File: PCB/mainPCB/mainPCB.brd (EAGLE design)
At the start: 187 x 85 mm, 129 parts, among them CN1 SDS-50J, CN2 SDS-50J, CN3 SDS-50J, CN4 SDS-50J, CN5 SDS-50J, CN6 SDS-50J, CN7 SDS-50J, CN8 SDS-50J, CON1 1776244-4, J2 RASPBERRYPI-40-PIN-GPIO, Q1 DMMT5401-7-F, T2 BC817, T3 BC817, T4 BC817, T5 BC817, T6 BC817, T7 BC817, T8 BC817, T9 BC817, U1 AT24C256C-SSHL-B, U11 SFH615A-07, U12 ALQ105, U13 SFH615A-07, U14 ALQ105, U15 SFH615A-07, U16 ALQ105, U17 SFH615A-07, U18 ALQ105, U19 SFH615A-07, U2 DMG2305UX-13SOT-23-M, U20 ALQ105, U3 SFH615A-07, U4 ALQ105, U5 SFH615A-07, U6 ALQ105, U7 SFH615A-07, U8 ALQ105

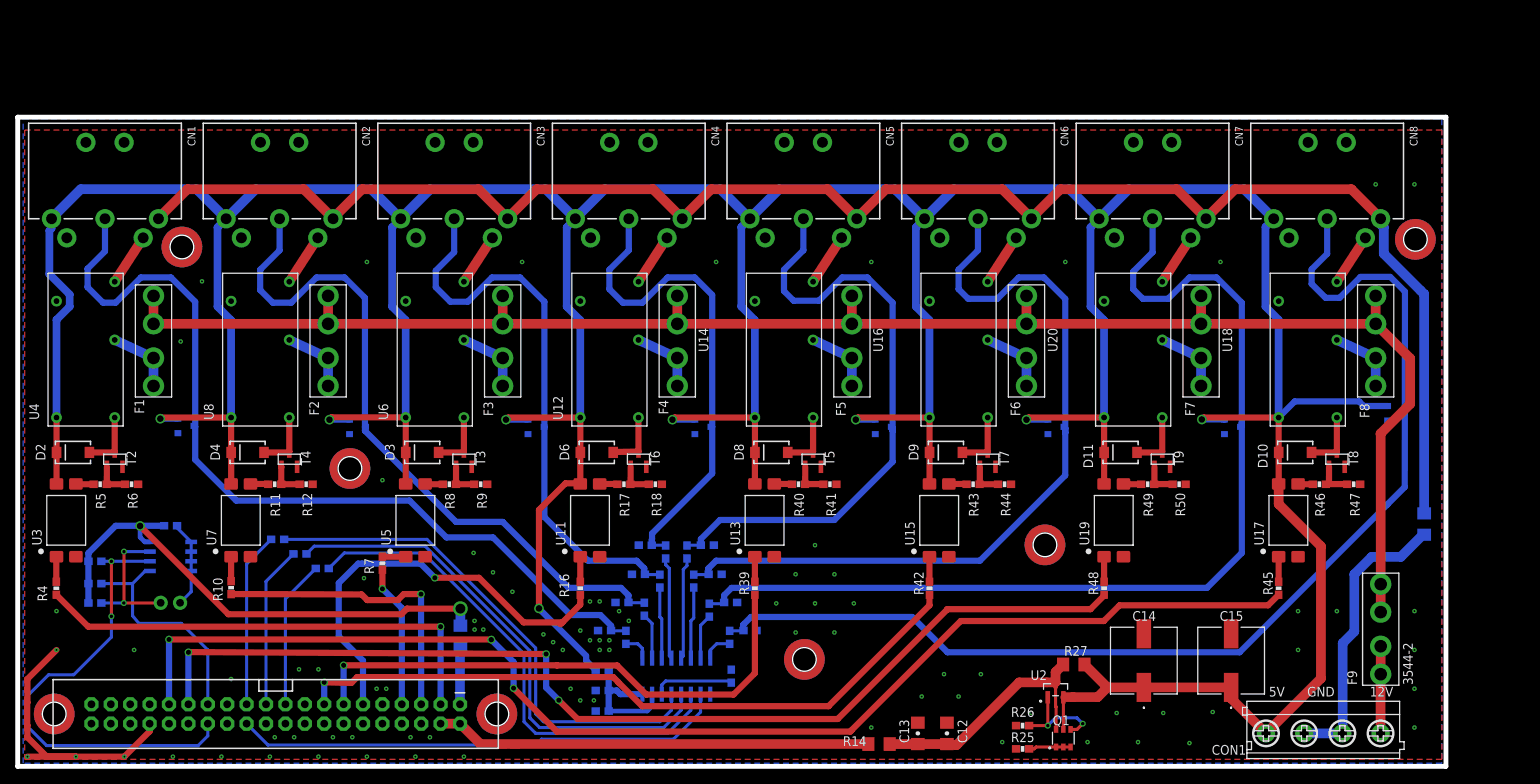
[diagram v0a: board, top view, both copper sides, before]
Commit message: Technically version 0.4. Sending it to JLCPCB for production.
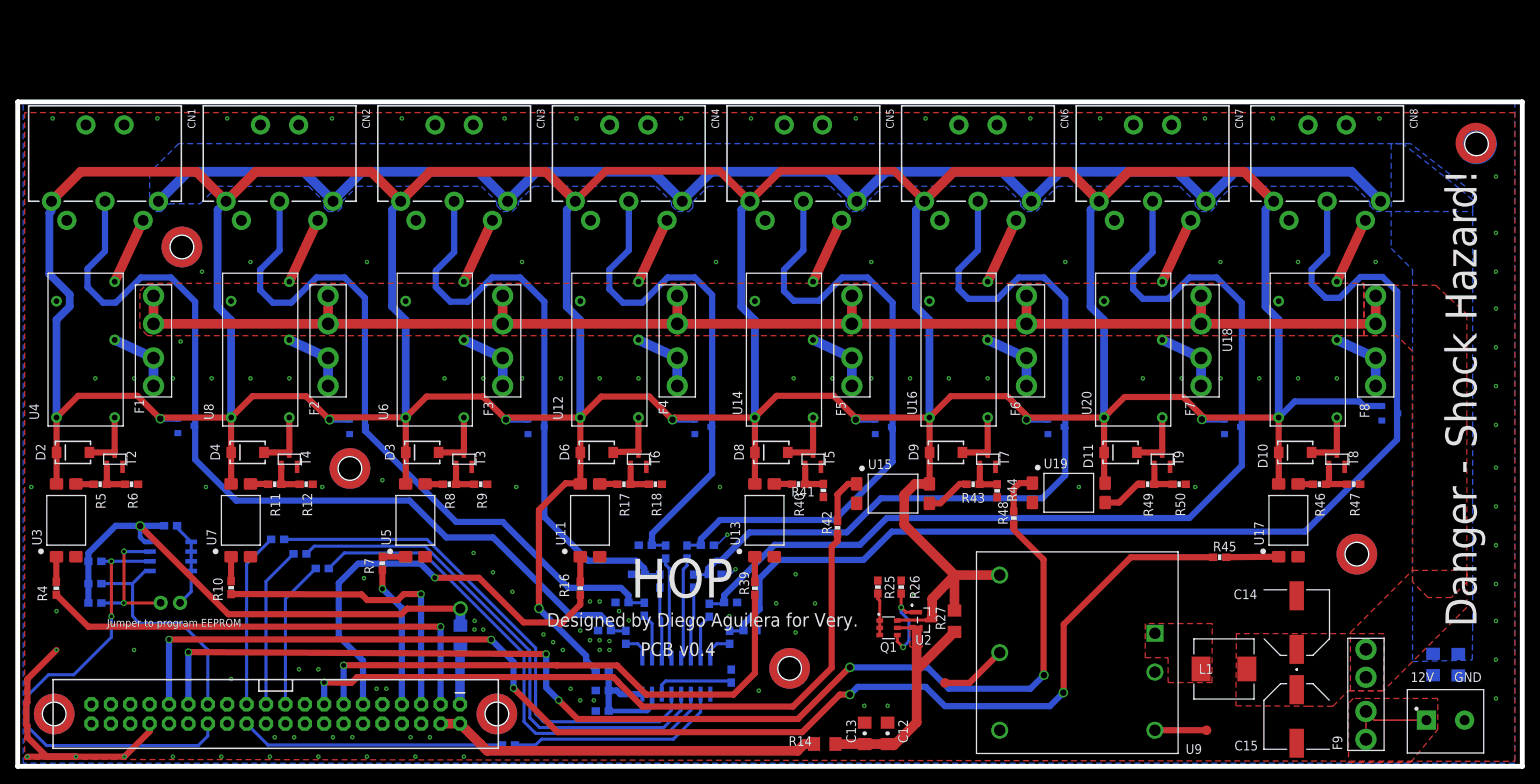
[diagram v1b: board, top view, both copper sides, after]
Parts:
- removed CON1: 1776244-4, lib:1776244-4
- added J1: 1935161, 1935161:PHOENIX_1935161
- added L1: DR73-1R0-R, DR73-1R0-R:DR73
- added R36: 0, SparkFun-Passives:1206
- added TP_ON/OFF, TP_TRIM: TEST-POINT3X5, SparkFun-Passives:PAD.03X.05
- added U9: S24SE05004PDFA, S24SE05004PDFA:CONV_S24SE05002PDFA
- C12, C13: value 10uF -> 1uF
- moved R25 28.4 mm to (112.6, 23.5), turned to 270 degrees
- moved Q1 27.1 mm to (114.0, 18.1), turned to 0 degrees
- moved R26 24.1 mm to (115.7, 23.5), turned to 270 degrees
- moved C14 20.6 mm to (167.5, 18.8)
- moved U2 19.6 mm to (118.6, 19.2), turned to 270 degrees
- moved R24 18.4 mm to (185.3, 13.3)
- moved R27 16.6 mm to (122.7, 19.0), turned to 270 degrees
- moved R48 15.0 mm to (130.4, 32.5)
- moved R42 14.4 mm to (107.3, 31.2)
- moved C15 11.3 mm to (167.5, 6.53), turned to 270 degrees
- moved F9 8.75 mm to (176.5, 9.42)
- moved R45 8.72 mm to (157.4, 27.4), turned to 0 degrees
- moved C12 7.77 mm to (113.9, 4.32)
- moved R14 7.11 mm to (105.7, 2.92)
- moved U15 6.98 mm to (114.6, 35.7), turned to 0 degrees
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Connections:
- removed net N$28: CON1.4, F9.P$1, F9.P$2
- new net N$30: TP_ON/OFF.P$1, U9.3
- new net N$52: L1.1, U9.1
- new net N$53: TP_TRIM.P$1, U9.5
- new net N$54: F9.P$1, F9.P$2, J1.1
- net 12V: now also C14.1, C15.1, L1.2
- net 5V: now also Q1.6, R27.1, U2.3, U9.6; no longer C14.1, C15.1, CON1.1, Q1.5, R27.2, U2.2
- net 5V_RPI: now also Q1.5, R27.2, U2.2; no longer Q1.6, R27.1, U2.3
- net COM: now also R36.1
- net GND: now also J1.2, R36.2, U9.2, U9.4; no longer CON1.2, CON1.3
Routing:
- net 5V: track 684.3 -> 770.4 mm
- net 12V: track 230.5 -> 189.3 mm
- net COM: track 223.5 -> 182.6 mm
- net GND: track 88.0 -> 54.9 mm, vias 86 -> 131
- net N$54: track 0.00 -> 12.0 mm
- net N$28: track 11.4 -> 0.00 mm
- net RELAY7: track 139.7 -> 151.0 mm, vias 3 -> 5
- net N$53: track 0.00 -> 8.80 mm
- net N$30: track 0.00 -> 6.76 mm
- net N$17: track 57.1 -> 50.7 mm
- net A7_F: track 133.9 -> 129.2 mm
- net N$41: track 2.33 -> 5.93 mm
- net N$44: track 3.27 -> 6.87 mm
- net A8_F: track 150.6 -> 147.1 mm
- net N$49: track 2.34 -> 5.76 mm
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- added copper zone on layer 1, net 12V
- added copper zone on layer 1, net 5V
- added copper zone on layer 1, net 5V_RPI
- added copper zone on layer 16, net COM
- added copper zone on layer 1, net N$52
- added copper zone on layer 1, net N$54
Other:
- board size 187 x 85 mm -> 197 x 87 mm
- board text added: "Danger - Shock Hazard!"
- board text added: "Designed by Diego Aguilera for Very."
- board text added: "HOP"
- board text added: "Jumper to program EEPROM"
- board text added: "PCB v0.4"
- board text removed: "5V"
- board text removed: "v0.3"
